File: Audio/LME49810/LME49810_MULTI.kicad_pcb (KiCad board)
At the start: 2 copper layers, 165.1 x 190.5 mm, 144 parts, among them P1 CONN_01X01, P10 CONN_01X01, P2 CONN_01X01, P3 CONN_01X01, P4 CONN_01X01, P5 CONN_01X01, P6 CONN_01X01, Q1 NPN(TO-3P-BCE), Q2 PNP(TO-3P-BCE), Q3 NPN(TO-220-BCE), U1 LME49810

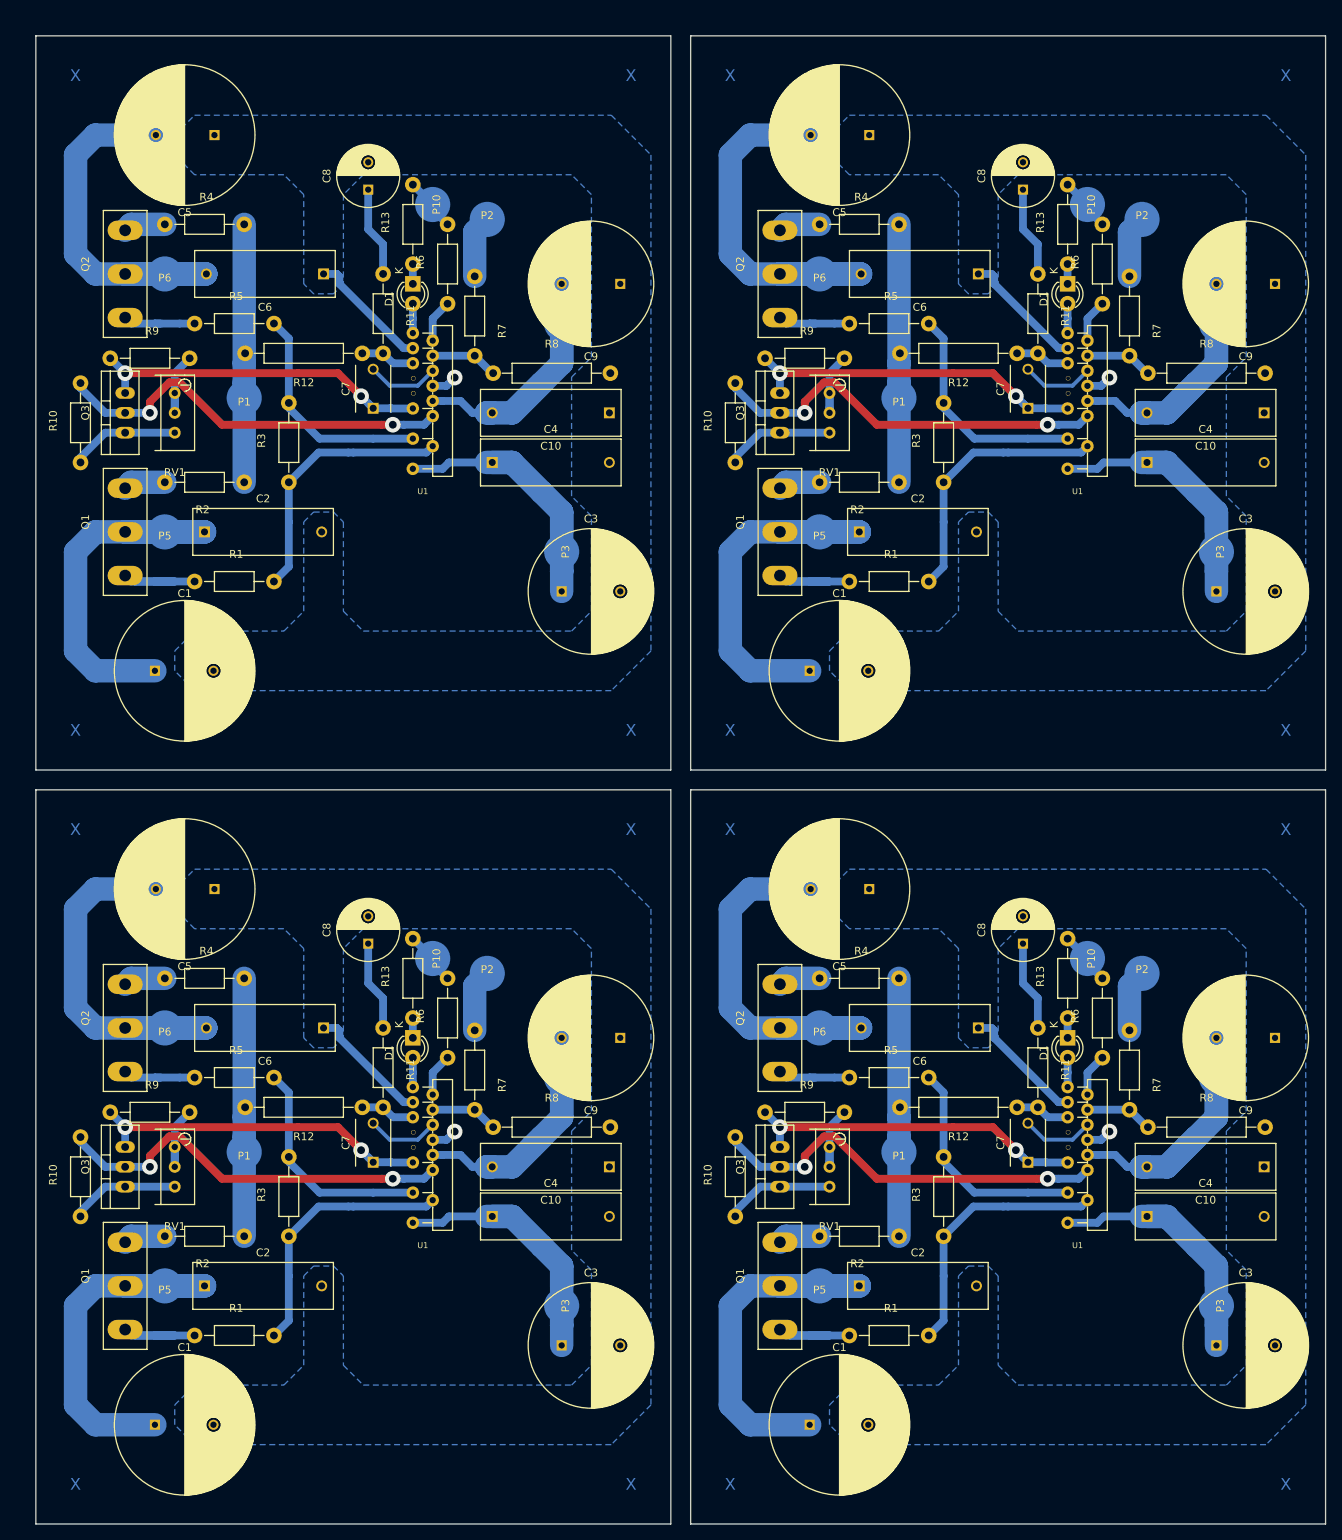
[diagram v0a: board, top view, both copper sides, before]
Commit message: Improvements
PCB revised.
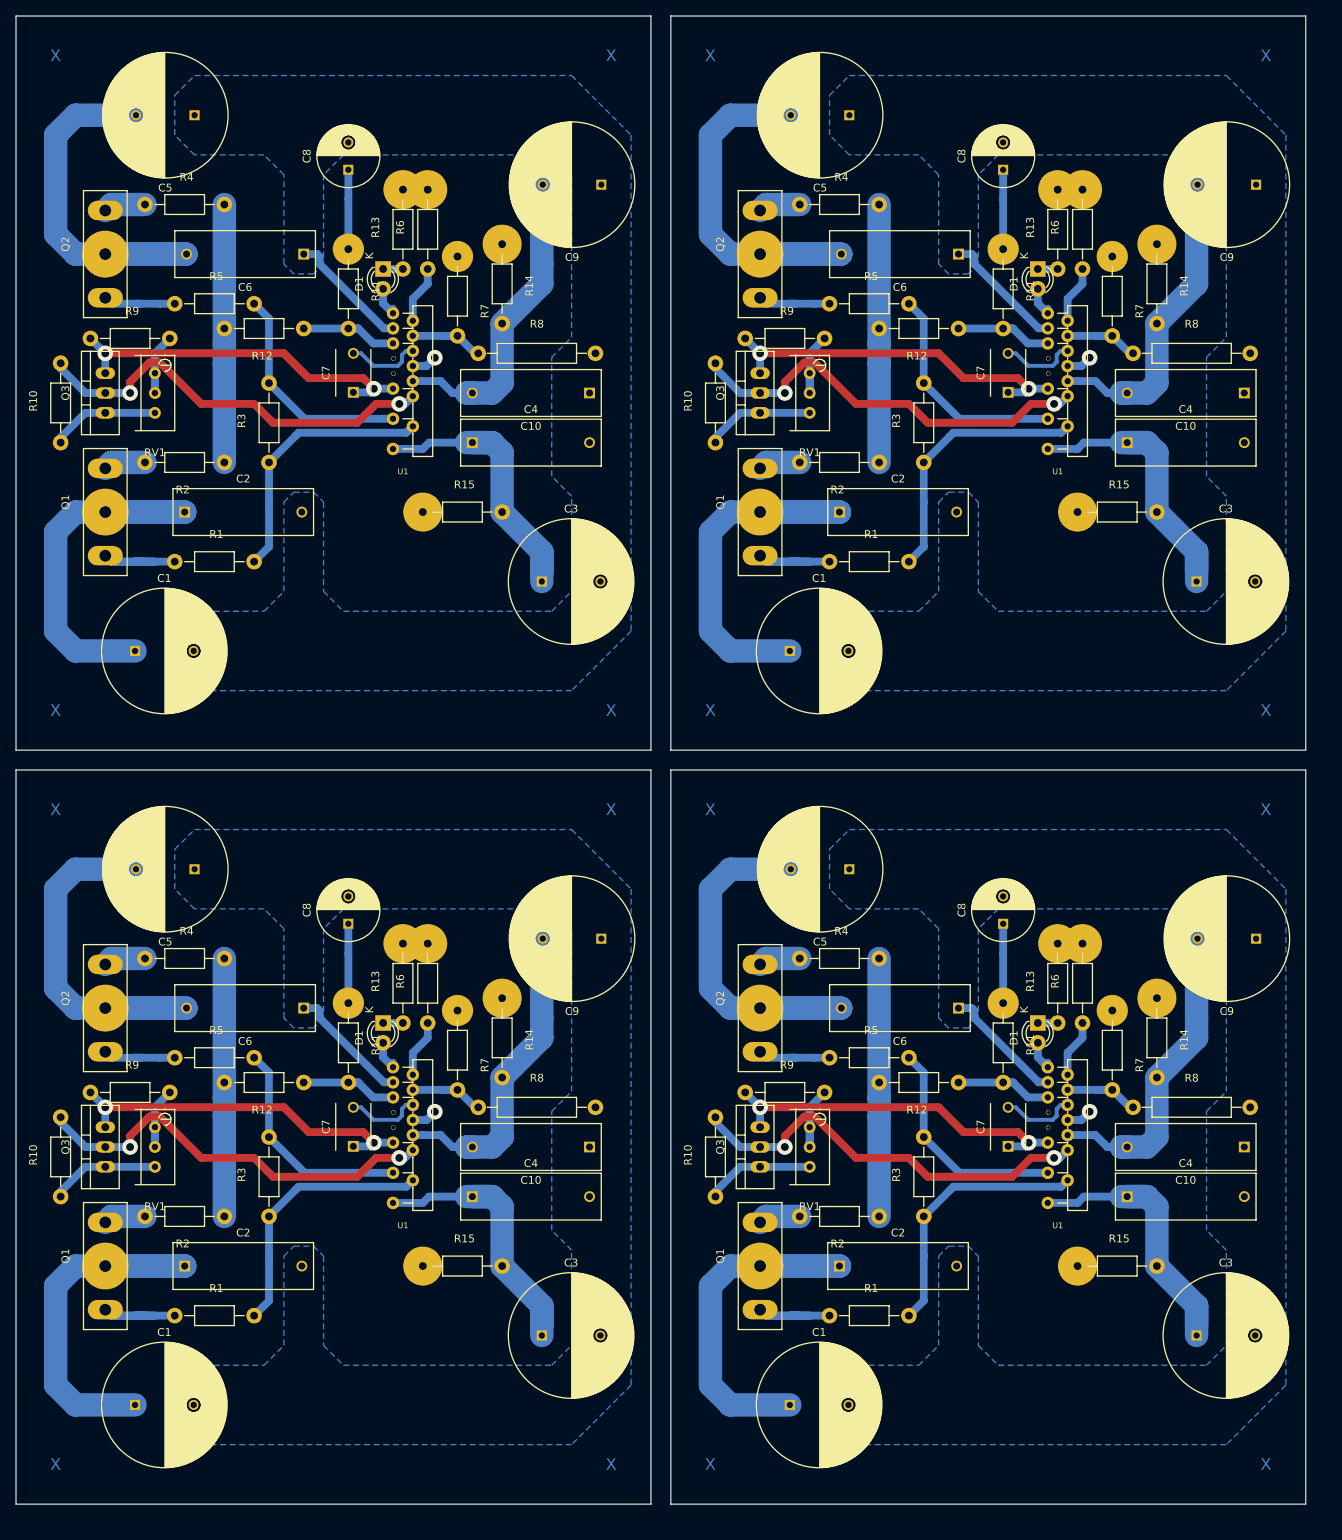
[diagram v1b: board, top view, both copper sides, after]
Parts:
- removed the C1 at (35.6, 101.6)
- removed the C1 at (119.4, 101.6)
- removed the C1 at (35.6, 198.1)
- removed the C1 at (119.4, 198.1)
- removed the C10 at (93.7, 68.6)
- removed the C10 at (177.6, 68.6)
- removed the C10 at (93.7, 165.1)
- removed the C10 at (177.6, 165.1)
- removed the C2 at (41.9, 83.8)
- removed the C2 at (125.7, 83.8)
- removed the C2 at (41.9, 180.3)
- removed the C2 at (125.7, 180.3)
- removed the C3 at (87.6, 91.4)
- removed the C3 at (171.4, 91.4)
- removed the C3 at (87.6, 188.0)
- removed the C3 at (171.4, 188.0)
- removed the C4 at (78.7, 74.9)
- removed the C4 at (162.6, 74.9)
- removed the C4 at (78.7, 171.4)
- removed the C4 at (162.6, 171.4)
- removed the C5 at (43.2, 33.0)
- removed the C5 at (127.0, 33.0)
- removed the C5 at (43.2, 129.5)
- removed the C5 at (127.0, 129.5)
- removed the C6 at (57.1, 50.8)
- removed the C6 at (141.0, 50.8)
- removed the C6 at (57.1, 147.3)
- removed the C6 at (141.0, 147.3)
- removed the C7 at (63.5, 68.0)
- removed the C7 at (147.3, 68.0)
- removed the C7 at (63.5, 164.5)
- removed the C7 at (147.3, 164.5)
- removed the C8 at (62.9, 40.0)
- removed the C8 at (146.7, 40.0)
- removed the C8 at (62.9, 136.5)
- removed the C8 at (146.7, 136.5)
- removed the C9 at (95.1, 52.1)
- removed the C9 at (178.9, 52.1)
- removed the C9 at (95.1, 148.6)
- removed the C9 at (178.9, 148.6)
- removed the D1 at (68.6, 52.1)
- removed the D1 at (152.4, 52.1)
- removed the D1 at (68.6, 148.6)
- removed the D1 at (152.4, 148.6)
- removed P1 (x4), P10 (x4), P2 (x4), P3 (x4), P4 (x4), P5 (x4), P6 (x4): CONN_01X01, LME49810:Soldering_pad
- removed the Q1 at (31.8, 83.8)
- removed the Q1 at (115.6, 83.8)
- removed the Q1 at (31.8, 180.3)
- removed the Q1 at (115.6, 180.3)
- removed the Q2 at (31.8, 50.8)
- removed the Q2 at (115.6, 50.8)
- removed the Q2 at (31.8, 147.3)
- removed the Q2 at (115.6, 147.3)
- removed the Q3 at (31.8, 68.6)
- removed the Q3 at (115.6, 68.6)
- removed the Q3 at (31.8, 165.1)
- removed the Q3 at (115.6, 165.1)
- removed the R1 at (45.7, 90.2)
- removed the R1 at (129.5, 90.2)
- removed the R1 at (45.7, 186.7)
- removed the R1 at (129.5, 186.7)
- removed the R10 at (26.0, 69.8)
- removed the R10 at (109.9, 69.8)
- removed the R10 at (26.0, 166.4)
- removed the R10 at (109.9, 166.4)
- removed the R11 at (64.8, 55.9)
- removed the R11 at (148.6, 55.9)
- removed the R11 at (64.8, 152.4)
- removed the R11 at (148.6, 152.4)
- removed the R12 at (54.6, 61.0)
- removed the R12 at (138.4, 61.0)
- removed the R12 at (54.6, 157.5)
- removed the R12 at (138.4, 157.5)
- removed the R13 at (68.6, 44.5)
- removed the R13 at (152.4, 44.5)
- removed the R13 at (68.6, 141.0)
- removed the R13 at (152.4, 141.0)
- removed the R2 at (41.9, 77.5)
- removed the R2 at (125.7, 77.5)
- removed the R2 at (41.9, 174.0)
- removed the R2 at (125.7, 174.0)
- removed the R3 at (52.7, 72.4)
- removed the R3 at (136.5, 72.4)
- removed the R3 at (52.7, 168.9)
- removed the R3 at (136.5, 168.9)
- removed the R4 at (41.9, 44.5)
- removed the R4 at (125.7, 44.5)
- removed the R4 at (41.9, 141.0)
- removed the R4 at (125.7, 141.0)
- removed the R5 at (45.7, 57.1)
- removed the R5 at (129.5, 57.1)
- removed the R5 at (45.7, 153.7)
- removed the R5 at (129.5, 153.7)
- removed the R6 at (73.0, 49.5)
- removed the R6 at (156.8, 49.5)
- removed the R6 at (73.0, 146.1)
- removed the R6 at (156.8, 146.1)
- removed the R7 at (76.5, 56.2)
- removed the R7 at (160.3, 56.2)
- removed the R7 at (76.5, 152.7)
- removed the R7 at (160.3, 152.7)
- removed the R8 at (86.4, 63.5)
- removed the R8 at (170.2, 63.5)
- removed the R8 at (86.4, 160.0)
- removed the R8 at (170.2, 160.0)
- removed the R9 at (34.9, 61.6)
- removed the R9 at (118.7, 61.6)
- removed the R9 at (34.9, 158.1)
- removed the R9 at (118.7, 158.1)
- removed the RV1 at (38.1, 66.0)
- removed the RV1 at (121.9, 66.0)
- removed the RV1 at (38.1, 162.6)
- removed the RV1 at (121.9, 162.6)
- removed the U1 at (69.8, 67.1)
- removed the U1 at (153.7, 67.1)
- removed the U1 at (69.8, 163.6)
- removed the U1 at (153.7, 163.6)
- added C1: 820u,100V, Capacitors_ThroughHole:C_Radial_D16_L31.5_P7.5, F.Cu at (33.0, 99.1)
- added C1: 820u,100V, Capacitors_ThroughHole:C_Radial_D16_L31.5_P7.5, F.Cu at (116.8, 99.1)
- added C1: 820u,100V, Capacitors_ThroughHole:C_Radial_D16_L31.5_P7.5, F.Cu at (33.0, 195.6)
- added C1: 820u,100V, Capacitors_ThroughHole:C_Radial_D16_L31.5_P7.5, F.Cu at (116.8, 195.6)
- added C10: 0.1u, Capacitors_ThroughHole:C_Rect_L18_W6_H12_P15, F.Cu at (91.2, 66.0)
- added C10: 0.1u, Capacitors_ThroughHole:C_Rect_L18_W6_H12_P15, F.Cu at (175.0, 66.0)
- added C10: 0.1u, Capacitors_ThroughHole:C_Rect_L18_W6_H12_P15, F.Cu at (91.2, 162.6)
- added C10: 0.1u, Capacitors_ThroughHole:C_Rect_L18_W6_H12_P15, F.Cu at (175.0, 162.6)
- added C2: 0.1u, Capacitors_ThroughHole:C_Rect_L18_W6_H12_P15, F.Cu at (39.4, 81.3)
- added C2: 0.1u, Capacitors_ThroughHole:C_Rect_L18_W6_H12_P15, F.Cu at (123.2, 81.3)
- added C2: 0.1u, Capacitors_ThroughHole:C_Rect_L18_W6_H12_P15, F.Cu at (39.4, 177.8)
- added C2: 0.1u, Capacitors_ThroughHole:C_Rect_L18_W6_H12_P15, F.Cu at (123.2, 177.8)
- added C3: 820u,100V, Capacitors_ThroughHole:C_Radial_D16_L31.5_P7.5, F.Cu at (85.1, 90.2)
- added C3: 820u,100V, Capacitors_ThroughHole:C_Radial_D16_L31.5_P7.5, F.Cu at (168.9, 90.2)
- added C3: 820u,100V, Capacitors_ThroughHole:C_Radial_D16_L31.5_P7.5, F.Cu at (85.1, 186.7)
- added C3: 820u,100V, Capacitors_ThroughHole:C_Radial_D16_L31.5_P7.5, F.Cu at (168.9, 186.7)
- added C4: 0.1u, Capacitors_ThroughHole:C_Rect_L18_W6_H12_P15, F.Cu at (76.2, 72.4)
- added C4: 0.1u, Capacitors_ThroughHole:C_Rect_L18_W6_H12_P15, F.Cu at (160.0, 72.4)
- added C4: 0.1u, Capacitors_ThroughHole:C_Rect_L18_W6_H12_P15, F.Cu at (76.2, 168.9)
- added C4: 0.1u, Capacitors_ThroughHole:C_Rect_L18_W6_H12_P15, F.Cu at (160.0, 168.9)
- added C5: 820u,100V, Capacitors_ThroughHole:C_Radial_D16_L31.5_P7.5, F.Cu at (40.6, 30.5)
- added C5: 820u,100V, Capacitors_ThroughHole:C_Radial_D16_L31.5_P7.5, F.Cu at (124.5, 30.5)
- added C5: 820u,100V, Capacitors_ThroughHole:C_Radial_D16_L31.5_P7.5, F.Cu at (40.6, 127.0)
- added C5: 820u,100V, Capacitors_ThroughHole:C_Radial_D16_L31.5_P7.5, F.Cu at (124.5, 127.0)
- added C6: 0.1u, Capacitors_ThroughHole:C_Rect_L18_W6_H12_P15, F.Cu at (54.6, 48.3)
- added C6: 0.1u, Capacitors_ThroughHole:C_Rect_L18_W6_H12_P15, F.Cu at (138.4, 48.3)
- added C6: 0.1u, Capacitors_ThroughHole:C_Rect_L18_W6_H12_P15, F.Cu at (54.6, 144.8)
- added C6: 0.1u, Capacitors_ThroughHole:C_Rect_L18_W6_H12_P15, F.Cu at (138.4, 144.8)
- added C7: 10p, Capacitors_ThroughHole:C_Disc_D6_P5, F.Cu at (61.0, 66.0)
- added C7: 10p, Capacitors_ThroughHole:C_Disc_D6_P5, F.Cu at (144.8, 66.0)
- added C7: 10p, Capacitors_ThroughHole:C_Disc_D6_P5, F.Cu at (61.0, 162.5)
- added C7: 10p, Capacitors_ThroughHole:C_Disc_D6_P5, F.Cu at (144.8, 162.5)
- added C8: 220u, Capacitors_ThroughHole:C_Radial_D8_L11.5_P3.5, F.Cu at (60.3, 37.5)
- added C8: 220u, Capacitors_ThroughHole:C_Radial_D8_L11.5_P3.5, F.Cu at (144.1, 37.5)
- added C8: 220u, Capacitors_ThroughHole:C_Radial_D8_L11.5_P3.5, F.Cu at (60.3, 134.0)
- added C8: 220u, Capacitors_ThroughHole:C_Radial_D8_L11.5_P3.5, F.Cu at (144.1, 134.0)
- added C9: 820u,100V, Capacitors_ThroughHole:C_Radial_D16_L31.5_P7.5, F.Cu at (92.7, 39.4)
- added C9: 820u,100V, Capacitors_ThroughHole:C_Radial_D16_L31.5_P7.5, F.Cu at (176.5, 39.4)
- added C9: 820u,100V, Capacitors_ThroughHole:C_Radial_D16_L31.5_P7.5, F.Cu at (92.7, 135.9)
- added C9: 820u,100V, Capacitors_ThroughHole:C_Radial_D16_L31.5_P7.5, F.Cu at (176.5, 135.9)
- added D1: LED, LEDs:LED-3MM, F.Cu at (64.8, 50.2)
- added D1: LED, LEDs:LED-3MM, F.Cu at (148.6, 50.2)
- added D1: LED, LEDs:LED-3MM, F.Cu at (64.8, 146.7)
- added D1: LED, LEDs:LED-3MM, F.Cu at (148.6, 146.7)
- added Q1: NPN(TO-3P-BCE), Transistors_TO-247:TO-247_Vertical_Neutral123, F.Cu at (29.2, 81.3)
- added Q1: NPN(TO-3P-BCE), Transistors_TO-247:TO-247_Vertical_Neutral123, F.Cu at (113.0, 81.3)
- added Q1: NPN(TO-3P-BCE), Transistors_TO-247:TO-247_Vertical_Neutral123, F.Cu at (29.2, 177.8)
- added Q1: NPN(TO-3P-BCE), Transistors_TO-247:TO-247_Vertical_Neutral123, F.Cu at (113.0, 177.8)
- added Q2: PNP(TO-3P-BCE), Transistors_TO-247:TO-247_Vertical_Neutral123, F.Cu at (29.2, 48.3)
- added Q2: PNP(TO-3P-BCE), Transistors_TO-247:TO-247_Vertical_Neutral123, F.Cu at (113.0, 48.3)
- added Q2: PNP(TO-3P-BCE), Transistors_TO-247:TO-247_Vertical_Neutral123, F.Cu at (29.2, 144.8)
- added Q2: PNP(TO-3P-BCE), Transistors_TO-247:TO-247_Vertical_Neutral123, F.Cu at (113.0, 144.8)
- added Q3: NPN(TO-220-BCE), Transistors_TO-220:TO-220_Neutral123_Vertical, F.Cu at (29.2, 66.0)
- added Q3: NPN(TO-220-BCE), Transistors_TO-220:TO-220_Neutral123_Vertical, F.Cu at (113.0, 66.0)
- added Q3: NPN(TO-220-BCE), Transistors_TO-220:TO-220_Neutral123_Vertical, F.Cu at (29.2, 162.6)
- added Q3: NPN(TO-220-BCE), Transistors_TO-220:TO-220_Neutral123_Vertical, F.Cu at (113.0, 162.6)
- added R1: 100, Resistors_ThroughHole:Resistor_Horizontal_RM10mm, F.Cu at (43.2, 87.6)
- added R1: 100, Resistors_ThroughHole:Resistor_Horizontal_RM10mm, F.Cu at (127.0, 87.6)
- added R1: 100, Resistors_ThroughHole:Resistor_Horizontal_RM10mm, F.Cu at (43.2, 184.2)
- added R1: 100, Resistors_ThroughHole:Resistor_Horizontal_RM10mm, F.Cu at (127.0, 184.2)
- added R10: 1.2k, Resistors_ThroughHole:Resistor_Horizontal_RM10mm, F.Cu at (23.5, 67.3)
- added R10: 1.2k, Resistors_ThroughHole:Resistor_Horizontal_RM10mm, F.Cu at (107.3, 67.3)
- added R10: 1.2k, Resistors_ThroughHole:Resistor_Horizontal_RM10mm, F.Cu at (23.5, 163.8)
- added R10: 1.2k, Resistors_ThroughHole:Resistor_Horizontal_RM10mm, F.Cu at (107.3, 163.8)
- added R11: 240, Resistors_ThroughHole:Resistor_Horizontal_RM10mm, F.Cu at (60.3, 52.7)
- added R11: 240, Resistors_ThroughHole:Resistor_Horizontal_RM10mm, F.Cu at (144.1, 52.7)
- added R11: 240, Resistors_ThroughHole:Resistor_Horizontal_RM10mm, F.Cu at (60.3, 149.2)
- added R11: 240, Resistors_ThroughHole:Resistor_Horizontal_RM10mm, F.Cu at (144.1, 149.2)
- added R12: 6.8k, Resistors_ThroughHole:Resistor_Horizontal_RM10mm, F.Cu at (49.5, 57.8)
- added R12: 6.8k, Resistors_ThroughHole:Resistor_Horizontal_RM10mm, F.Cu at (133.3, 57.8)
- added R12: 6.8k, Resistors_ThroughHole:Resistor_Horizontal_RM10mm, F.Cu at (49.5, 154.3)
- added R12: 6.8k, Resistors_ThroughHole:Resistor_Horizontal_RM10mm, F.Cu at (133.3, 154.3)
- added R13: 470, Resistors_ThroughHole:Resistor_Horizontal_RM10mm, F.Cu at (67.3, 45.1)
- added R13: 470, Resistors_ThroughHole:Resistor_Horizontal_RM10mm, F.Cu at (151.1, 45.1)
- added R13: 470, Resistors_ThroughHole:Resistor_Horizontal_RM10mm, F.Cu at (67.3, 141.6)
- added R13: 470, Resistors_ThroughHole:Resistor_Horizontal_RM10mm, F.Cu at (151.1, 141.6)
- added R14: 10, Resistors_ThroughHole:Resistor_Horizontal_RM10mm, F.Cu at (80.0, 52.1)
- added R14: 10, Resistors_ThroughHole:Resistor_Horizontal_RM10mm, F.Cu at (163.8, 52.1)
- added R14: 10, Resistors_ThroughHole:Resistor_Horizontal_RM10mm, F.Cu at (80.0, 148.6)
- added R14: 10, Resistors_ThroughHole:Resistor_Horizontal_RM10mm, F.Cu at (163.8, 148.6)
- added R15: 10, Resistors_ThroughHole:Resistor_Horizontal_RM10mm, F.Cu at (74.9, 81.3)
- added R15: 10, Resistors_ThroughHole:Resistor_Horizontal_RM10mm, F.Cu at (158.8, 81.3)
- added R15: 10, Resistors_ThroughHole:Resistor_Horizontal_RM10mm, F.Cu at (74.9, 177.8)
- added R15: 10, Resistors_ThroughHole:Resistor_Horizontal_RM10mm, F.Cu at (158.8, 177.8)
- added R2: 0.22, Resistors_ThroughHole:Resistor_Horizontal_RM10mm, F.Cu at (39.4, 74.9)
- added R2: 0.22, Resistors_ThroughHole:Resistor_Horizontal_RM10mm, F.Cu at (123.2, 74.9)
- added R2: 0.22, Resistors_ThroughHole:Resistor_Horizontal_RM10mm, F.Cu at (39.4, 171.4)
- added R2: 0.22, Resistors_ThroughHole:Resistor_Horizontal_RM10mm, F.Cu at (123.2, 171.4)
- added R3: 2.2k, Resistors_ThroughHole:Resistor_Horizontal_RM10mm, F.Cu at (50.2, 69.8)
- added R3: 2.2k, Resistors_ThroughHole:Resistor_Horizontal_RM10mm, F.Cu at (134.0, 69.8)
- added R3: 2.2k, Resistors_ThroughHole:Resistor_Horizontal_RM10mm, F.Cu at (50.2, 166.4)
- added R3: 2.2k, Resistors_ThroughHole:Resistor_Horizontal_RM10mm, F.Cu at (134.0, 166.4)
- added R4: 0.22, Resistors_ThroughHole:Resistor_Horizontal_RM10mm, F.Cu at (39.4, 41.9)
- added R4: 0.22, Resistors_ThroughHole:Resistor_Horizontal_RM10mm, F.Cu at (123.2, 41.9)
- added R4: 0.22, Resistors_ThroughHole:Resistor_Horizontal_RM10mm, F.Cu at (39.4, 138.4)
- added R4: 0.22, Resistors_ThroughHole:Resistor_Horizontal_RM10mm, F.Cu at (123.2, 138.4)
- added R5: 100, Resistors_ThroughHole:Resistor_Horizontal_RM10mm, F.Cu at (43.2, 54.6)
- added R5: 100, Resistors_ThroughHole:Resistor_Horizontal_RM10mm, F.Cu at (127.0, 54.6)
- added R5: 100, Resistors_ThroughHole:Resistor_Horizontal_RM10mm, F.Cu at (43.2, 151.1)
- added R5: 100, Resistors_ThroughHole:Resistor_Horizontal_RM10mm, F.Cu at (127.0, 151.1)
- added R6: 33k, Resistors_ThroughHole:Resistor_Horizontal_RM10mm, F.Cu at (70.5, 45.1)
- added R6: 33k, Resistors_ThroughHole:Resistor_Horizontal_RM10mm, F.Cu at (154.3, 45.1)
- added R6: 33k, Resistors_ThroughHole:Resistor_Horizontal_RM10mm, F.Cu at (70.5, 141.6)
- added R6: 33k, Resistors_ThroughHole:Resistor_Horizontal_RM10mm, F.Cu at (154.3, 141.6)
- added R7: 240, Resistors_ThroughHole:Resistor_Horizontal_RM10mm, F.Cu at (74.3, 53.6)
- added R7: 240, Resistors_ThroughHole:Resistor_Horizontal_RM10mm, F.Cu at (158.1, 53.6)
- added R7: 240, Resistors_ThroughHole:Resistor_Horizontal_RM10mm, F.Cu at (74.3, 150.2)
- added R7: 240, Resistors_ThroughHole:Resistor_Horizontal_RM10mm, F.Cu at (158.1, 150.2)
- added R8: 6.8k, Resistors_ThroughHole:Resistor_Horizontal_RM15mm, F.Cu at (84.5, 61.0)
- added R8: 6.8k, Resistors_ThroughHole:Resistor_Horizontal_RM15mm, F.Cu at (168.3, 61.0)
- added R8: 6.8k, Resistors_ThroughHole:Resistor_Horizontal_RM15mm, F.Cu at (84.5, 157.5)
- added R8: 6.8k, Resistors_ThroughHole:Resistor_Horizontal_RM15mm, F.Cu at (168.3, 157.5)
- added R9: 360, Resistors_ThroughHole:Resistor_Horizontal_RM10mm, F.Cu at (32.4, 59.1)
- added R9: 360, Resistors_ThroughHole:Resistor_Horizontal_RM10mm, F.Cu at (116.2, 59.1)
- added R9: 360, Resistors_ThroughHole:Resistor_Horizontal_RM10mm, F.Cu at (32.4, 155.6)
- added R9: 360, Resistors_ThroughHole:Resistor_Horizontal_RM10mm, F.Cu at (116.2, 155.6)
- added RV1: 200, Potentiometers:Potentiometer_Bourns_3296W_3-8Zoll_Inline_ScrewUp, F.Cu at (35.6, 63.5)
- added RV1: 200, Potentiometers:Potentiometer_Bourns_3296W_3-8Zoll_Inline_ScrewUp, F.Cu at (119.4, 63.5)
- added RV1: 200, Potentiometers:Potentiometer_Bourns_3296W_3-8Zoll_Inline_ScrewUp, F.Cu at (35.6, 160.0)
- added RV1: 200, Potentiometers:Potentiometer_Bourns_3296W_3-8Zoll_Inline_ScrewUp, F.Cu at (119.4, 160.0)
- added U1: LME49810, LME49810:LME49810, F.Cu at (67.3, 64.5)
- added U1: LME49810, LME49810:LME49810, F.Cu at (151.1, 64.5)
- added U1: LME49810, LME49810:LME49810, F.Cu at (67.3, 161.0)
- added U1: LME49810, LME49810:LME49810, F.Cu at (151.1, 161.0)
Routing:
- net -VeeL1: track 164.6 -> 0.00 mm
- net Net-(C10-Pad2): track 0.00 -> 163.3 mm
- net +VccL1: track 159.2 -> 0.00 mm
- net Net-(C3-Pad1): track 0.00 -> 154.1 mm
- net /InputLH: track 31.8 -> 0.00 mm
- net Net-(R11-Pad2): track 27.5 -> 54.0 mm
- net /Emit-PNP: track 21.6 -> 0.00 mm
- net /Emit-NPN: track 21.6 -> 0.00 mm
- net Net-(Q2-Pad3): track 0.00 -> 21.6 mm
- net Net-(Q1-Pad3): track 0.00 -> 21.6 mm
- net +5V: track 27.7 -> 12.7 mm
- net ELH: track 175.7 -> 187.1 mm
- net Net-(R7-Pad2): track 34.7 -> 43.4 mm
- net Net-(R6-Pad1): track 22.1 -> 29.7 mm
- net CLH: track 208.7 -> 216.3 mm
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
